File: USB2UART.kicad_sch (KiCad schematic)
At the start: 12 parts, among them J1 Conn_01x04, J2 Conn_01x03, J3 Conn_01x03, J4 Conn_01x02, J5 Conn_01x02

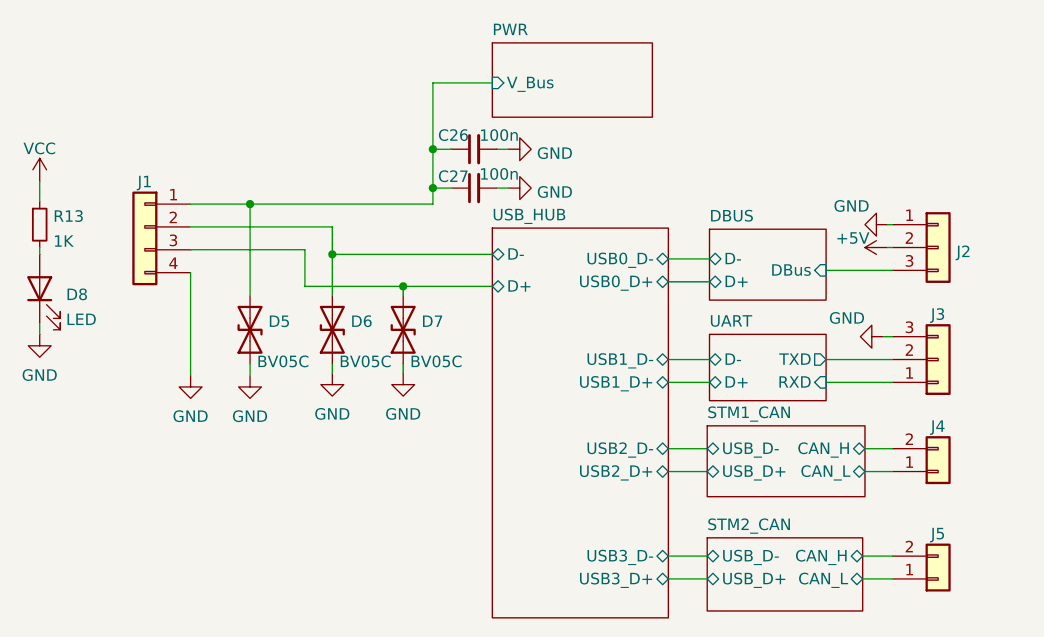
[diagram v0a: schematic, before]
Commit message: USB2UART
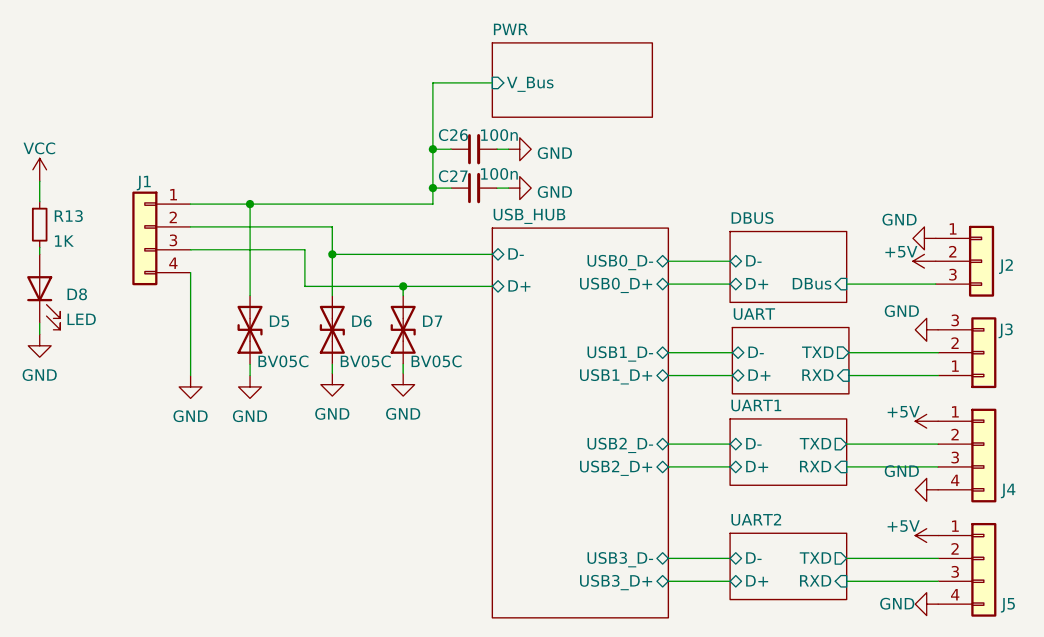
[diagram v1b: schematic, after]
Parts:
- removed J4, J5: Conn_01x02, Connector_JST:JST_GH_SM02B-GHS-TB_1x02-1MP_P1.25mm_Horizontal, symbol Connector_Generic:Conn_01x02
- added J4, J5: Conn_01x03, Connector_JST:JST_GH_SM04B-GHS-TB_1x04-1MP_P1.25mm_Horizontal, symbol Connector_Generic:Conn_01x04
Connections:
- net +5V: now also J4.1 (Pin_1), J5.1 (Pin_1)
- net GND: now also J4.4 (Pin_4), J5.4 (Pin_4)
- new net UART1/RXD: J4.3 (Pin_3)
- new net UART1/TXD: J4.2 (Pin_2)
- new net UART2/RXD: J5.3 (Pin_3)
- new net UART2/TXD: J5.2 (Pin_2)
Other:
- removed sheet STM1_CAN
- removed sheet STM2_CAN
- added sheet UART1 (subsch/UART.kicad_sch)
- added sheet UART2 (subsch/UART.kicad_sch)
- moved on the sheet: J2, J3

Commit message: another right version
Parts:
- J4, J5: value Conn_01x03 -> Conn_01x04
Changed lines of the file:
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@@
     (in_bom yes) (on_board yes)
     (property "Reference" "J5" (id 0) (at 180.594 127 0))
-    (property "Value" "Conn_01x03" (id 1) (at 179.832 123.7866 0)
+    (property "Value" "Conn_01x04" (id 1) (at 179.832 123.7866 0)
       (effects (font (size 1.27 1.27)) (justify left) hide)
     )
@@
     (in_bom yes) (on_board yes)
     (property "Reference" "J4" (id 0) (at 180.594 114.3 0))
-    (property "Value" "Conn_01x03" (id 1) (at 179.832 111.0866 0)
+    (property "Value" "Conn_01x04" (id 1) (at 179.832 111.0866 0)
       (effects (font (size 1.27 1.27)) (justify left) hide)
     )
@@
     )
     (path "/d5c10d34-5ae0-4a6b-bad8-d4ed4b393fc8"
-      (reference "J4") (unit 1) (value "Conn_01x03") (footprint "Connector_JST:JST_GH_SM04B-GHS-TB_1x04-1MP_P1.25mm_Horizontal")
+      (reference "J4") (unit 1) (value "Conn_01x04") (footprint "Connector_JST:JST_GH_SM04B-GHS-TB_1x04-1MP_P1.25mm_Horizontal")
     )
     (path "/5c0ed9d4-4fd9-4462-8972-42835e322755"
-      (reference "J5") (unit 1) (value "Conn_01x03") (footprint "Connector_JST:JST_GH_SM04B-GHS-TB_1x04-1MP_P1.25mm_Horizontal")
+      (reference "J5") (unit 1) (value "Conn_01x04") (footprint "Connector_JST:JST_GH_SM04B-GHS-TB_1x04-1MP_P1.25mm_Horizontal")
     )
     (path "/71b07c00-0314-4dfd-92cb-aca2c9812e1b/e5588e62-caec-4581-8753-afa8055836e7"
